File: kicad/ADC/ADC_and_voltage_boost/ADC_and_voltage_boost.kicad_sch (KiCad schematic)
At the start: 10 parts, among them J1 Screw_Terminal_01x04, J4 Screw_Terminal_01x02, U3 MOUDLE-SEEEDUINO-XIAO-ESP32C3, U4 MAX1032BEUG_

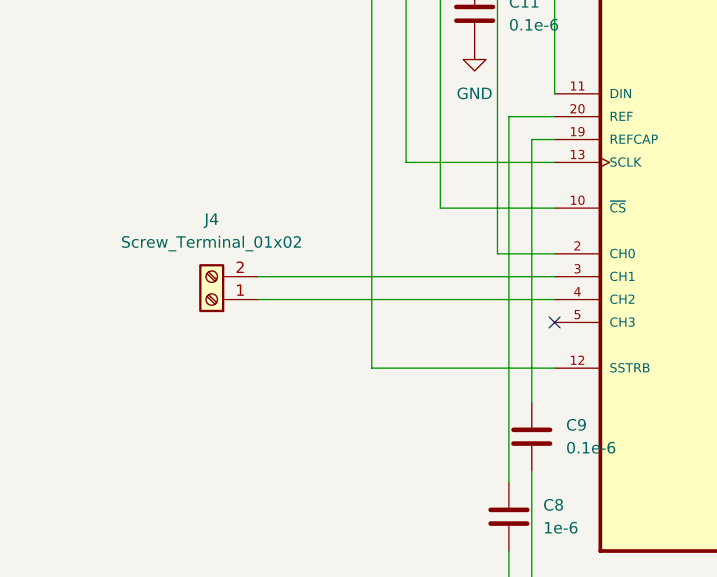
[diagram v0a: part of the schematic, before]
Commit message: updated pcb
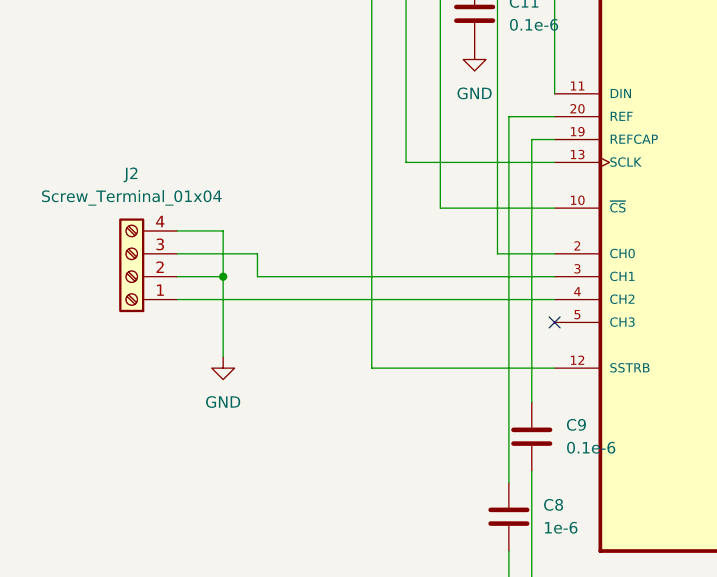
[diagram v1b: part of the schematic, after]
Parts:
- removed J4: Screw_Terminal_01x02, TerminalBlock_Phoenix:TerminalBlock_Phoenix_MPT-0,5-2-2.54_1x02_P2.54mm_Horizontal, symbol Connector:Screw_Terminal_01x02
- added J2: Screw_Terminal_01x04, TerminalBlock_Phoenix:TerminalBlock_Phoenix_MPT-0,5-4-2.54_1x04_P2.54mm_Horizontal, symbol Connector:Screw_Terminal_01x04
- C1, C11, C2, C3, C8, C9: footprint Capacitor_SMD:C_1206_3216Metric_Pad1.33x1.80mm_HandSolder -> Capacitor_SMD:C_0805_2012Metric
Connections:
- net GND: now also J2.2 (Pin_2), J2.4 (Pin_4)
- net at U4.3 (CH1): now also J2.3 (Pin_3)
- net at U4.4 (CH2): now also J2.1 (Pin_1)
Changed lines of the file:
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@@
+	)
+	(junction
+		(at 88.9 118.11)
+		(diameter 0)
+		(color 0 0 0 0)
 	)
 	(junction
@@
 	(wire
 		(pts
+			(xy 83.82 118.11) (xy 88.9 118.11)
+		)
+		(stroke
+			(width 0)
+			(type default)
+		)
+	)
+	(wire
+		(pts
 			(xy 161.29 87.63) (xy 191.77 87.63)
 		)
@@
 	(wire
 		(pts
+			(xy 88.9 118.11) (xy 88.9 127)
+		)
+		(stroke
+			(width 0)
+			(type default)
+		)
+	)
+	(wire
+		(pts
 			(xy 119.38 85.09) (xy 116.84 85.09)
 		)
@@
 	(wire
 		(pts
+			(xy 83.82 115.57) (xy 92.71 115.57)
+		)
+		(stroke
+			(width 0)
+			(type default)
+		)
+	)
+	(wire
+		(pts
+			(xy 83.82 120.65) (xy 125.73 120.65)
+		)
+		(stroke
+			(width 0)
+			(type default)
+		)
+	)
+	(wire
+		(pts
 			(xy 113.03 110.49) (xy 113.03 33.02)
 		)
@@
 	(wire
 		(pts
-			(xy 125.73 120.65) (xy 92.71 120.65)
-		)
-		(stroke
-			(width 0)
-			(type default)
-		)
-	)
-	(wire
-		(pts
 			(xy 166.37 74.93) (xy 166.37 92.71)
 		)
@@
 	(wire
 		(pts
+			(xy 83.82 113.03) (xy 88.9 113.03)
+		)
+		(stroke
+			(width 0)
+			(type default)
+		)
+	)
+	(wire
+		(pts
 			(xy 125.73 118.11) (xy 92.71 118.11)
 		)
@@
 	(wire
 		(pts
+			(xy 92.71 118.11) (xy 92.71 115.57)
+		)
+		(stroke
+			(width 0)
+			(type default)
+		)
+	)
+	(wire
+		(pts
 			(xy 119.38 74.93) (xy 166.37 74.93)
+		)
+		(stroke
+			(width 0)
+			(type default)
+		)
+	)
+	(wire
+		(pts
+			(xy 88.9 113.03) (xy 88.9 118.11)
 		)
 		(stroke
@@
 			)
 		)
-		(property "Footprint" "Capacitor_SMD:C_1206_3216Metric_Pad1.33x1.80mm_HandSolder"
+		(property "Footprint" "Capacitor_SMD:C_0805_2012Metric"
 			(at 182.5752 97.79 0)
 			(effects
@@
 			)
 		)
-		(property "Footprint" "Capacitor_SMD:C_1206_3216Metric_Pad1.33x1.80mm_HandSolder"
+		(property "Footprint" "Capacitor_SMD:C_0805_2012Metric"
 			(at 119.6848 140.97 0)
 			(effects
@@
 	)
 	(symbol
+		(lib_id "Connector:Screw_Terminal_01x04")
+		(at 78.74 118.11 180)
+		(unit 1)
+		(exclude_from_sim no)
+		(in_bom yes)
+		(on_board yes)
+		(dnp no)
+		(fields_autoplaced yes)
+		(property "Reference" "J2"
+			(at 78.74 106.68 0)
+			(effects
+				(font
+					(size 1.27 1.27)
+				)
+			)
+		)
+		(property "Value" "Screw_Terminal_01x04"
+			(at 78.74 109.22 0)
+			(effects
+				(font
+					(size 1.27 1.27)
+				)
+			)
+		)
+		(property "Footprint" "TerminalBlock_Phoenix:TerminalBlock_Phoenix_MPT-0,5-4-2.54_1x04_P2.54mm_Horizontal"
+			(at 78.74 118.11 0)
+			(effects
+				(font
+					(size 1.27 1.27)
+				)
+				(hide yes)
+			)
+		)
+		(property "Datasheet" "~"
+			(at 78.74 118.11 0)
+			(effects
+				(font
+					(size 1.27 1.27)
+				)
+				(hide yes)
+			)
+		)
+		(property "Description" "Generic screw terminal, single row, 01x04, script generated (kicad-library-utils/schlib/autogen/connector/)"
+			(at 78.74 118.11 0)
+			(effects
+				(font
+					(size 1.27 1.27)
+				)
+				(hide yes)
+			)
+		)
+		(pin "1"
+		)
+		(pin "2"
+		)
+		(pin "3"
+		)
+		(pin "4"
+		)
+		(instances
+			(project "ADC_and_voltage_boost"
+				(path "/47c680de-131f-4b08-bf1d-2ba63acc97af"
+					(reference "J2")
+					(unit 1)
+				)
+			)
+		)
+	)
+	(symbol
 		(lib_id "power:+3.3V")
 		(at 176.53 40.64 0)
@@
 			)
 		)
-		(property "Footprint" "Capacitor_SMD:C_1206_3216Metric_Pad1.33x1.80mm_HandSolder"
+		(property "Footprint" "Capacitor_SMD:C_0805_2012Metric"
 			(at 204.1652 92.71 0)
 			(effects
@@
 			)
 		)
-		(property "Footprint" "Capacitor_SMD:C_1206_3216Metric_Pad1.33x1.80mm_HandSolder"
+		(property "Footprint" "Capacitor_SMD:C_0805_2012Metric"
 			(at 117.8052 92.71 0)
 			(effects
@@
 	)
 	(symbol
-		(lib_id "Connector:Screw_Terminal_01x02")
-		(at 87.63 120.65 180)
-		(unit 1)
-		(exclude_from_sim no)
-		(in_bom yes)
-		(on_board yes)
-		(dnp no)
-		(fields_autoplaced yes)
-		(property "Reference" "J4"
-			(at 87.63 111.76 0)
-			(effects
-				(font
-					(size 1.27 1.27)
-				)
-			)
-		)
-		(property "Value" "Screw_Terminal_01x02"
-			(at 87.63 114.3 0)
-			(effects
-				(font
-					(size 1.27 1.27)
-				)
-			)
-		)
-		(property "Footprint" "TerminalBlock_Phoenix:TerminalBlock_Phoenix_MPT-0,5-2-2.54_1x02_P2.54mm_Horizontal"
-			(at 87.63 120.65 0)
-			(effects
-				(font
-					(size 1.27 1.27)
-				)
-				(hide yes)
-			)
-		)
-		(property "Datasheet" "~"
-			(at 87.63 120.65 0)
-			(effects
-				(font
-					(size 1.27 1.27)
-				)
-				(hide yes)
-			)
-		)
-		(property "Description" "Generic screw terminal, single row, 01x02, script generated (kicad-library-utils/schlib/autogen/connector/)"
-			(at 87.63 120.65 0)
-			(effects
-				(font
-					(size 1.27 1.27)
-				)
-				(hide yes)
-			)
-		)
-		(pin "2"
-		)
-		(pin "1"
-		)
-		(instances
-			(project "ADC_and_voltage_boost"
-				(path "/47c680de-131f-4b08-bf1d-2ba63acc97af"
-					(reference "J4")
-					(unit 1)
-				)
-			)
-		)
-	)
-	(symbol
 		(lib_id "power:+5V")
 		(at 166.37 92.71 270)
@@
 	(symbol
 		(lib_id "power:GND")
+		(at 88.9 127 0)
+		(unit 1)
+		(exclude_from_sim no)
+		(in_bom yes)
+		(on_board yes)
+		(dnp no)
+		(fields_autoplaced yes)
+		(property "Reference" "#PWR012"
+			(at 88.9 133.35 0)
+			(effects
+				(font
+					(size 1.27 1.27)
+				)
+				(hide yes)
+			)
+		)
+		(property "Value" "GND"
+			(at 88.9 132.08 0)
+			(effects
+				(font
+					(size 1.27 1.27)
+				)
+			)
+		)
+		(property "Footprint" ""
+			(at 88.9 127 0)
+			(effects
+				(font
+					(size 1.27 1.27)
+				)
+				(hide yes)
+			)
+		)
+		(property "Datasheet" ""
+			(at 88.9 127 0)
+			(effects
+				(font
+					(size 1.27 1.27)
+				)
+				(hide yes)
+			)
+		)
+		(property "Description" ""
+			(at 88.9 127 0)
+			(effects
+				(font
+					(size 1.27 1.27)
+				)
+			)
+		)
+		(pin "1"
+		)
+		(instances
+			(project "ADC_and_voltage_boost"
+				(path "/47c680de-131f-4b08-bf1d-2ba63acc97af"
+					(reference "#PWR012")
+					(unit 1)
+				)
+			)
+		)
+	)
+	(symbol
+		(lib_id "power:GND")
 		(at 116.84 92.71 0)
 		(unit 1)
@@
 			)
 		)
-		(property "Footprint" "Capacitor_SMD:C_1206_3216Metric_Pad1.33x1.80mm_HandSolder"
+		(property "Footprint" "Capacitor_SMD:C_0805_2012Metric"
 			(at 195.2752 97.79 0)
 			(effects
@@
 			)
 		)
-		(property "Footprint" "Capacitor_SMD:C_1206_3216Metric_Pad1.33x1.80mm_HandSolder"
+		(property "Footprint" "Capacitor_SMD:C_0805_2012Metric"
 			(at 122.2248 132.08 0)
 			(effects
